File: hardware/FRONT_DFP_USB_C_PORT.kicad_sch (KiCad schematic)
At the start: 26 parts, among them J5 USB4200-03-A (VIRT FLAG MOUNT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, Q18 PMOS, Q19 PMOS, Q20 PMOS, Q21 PMOS

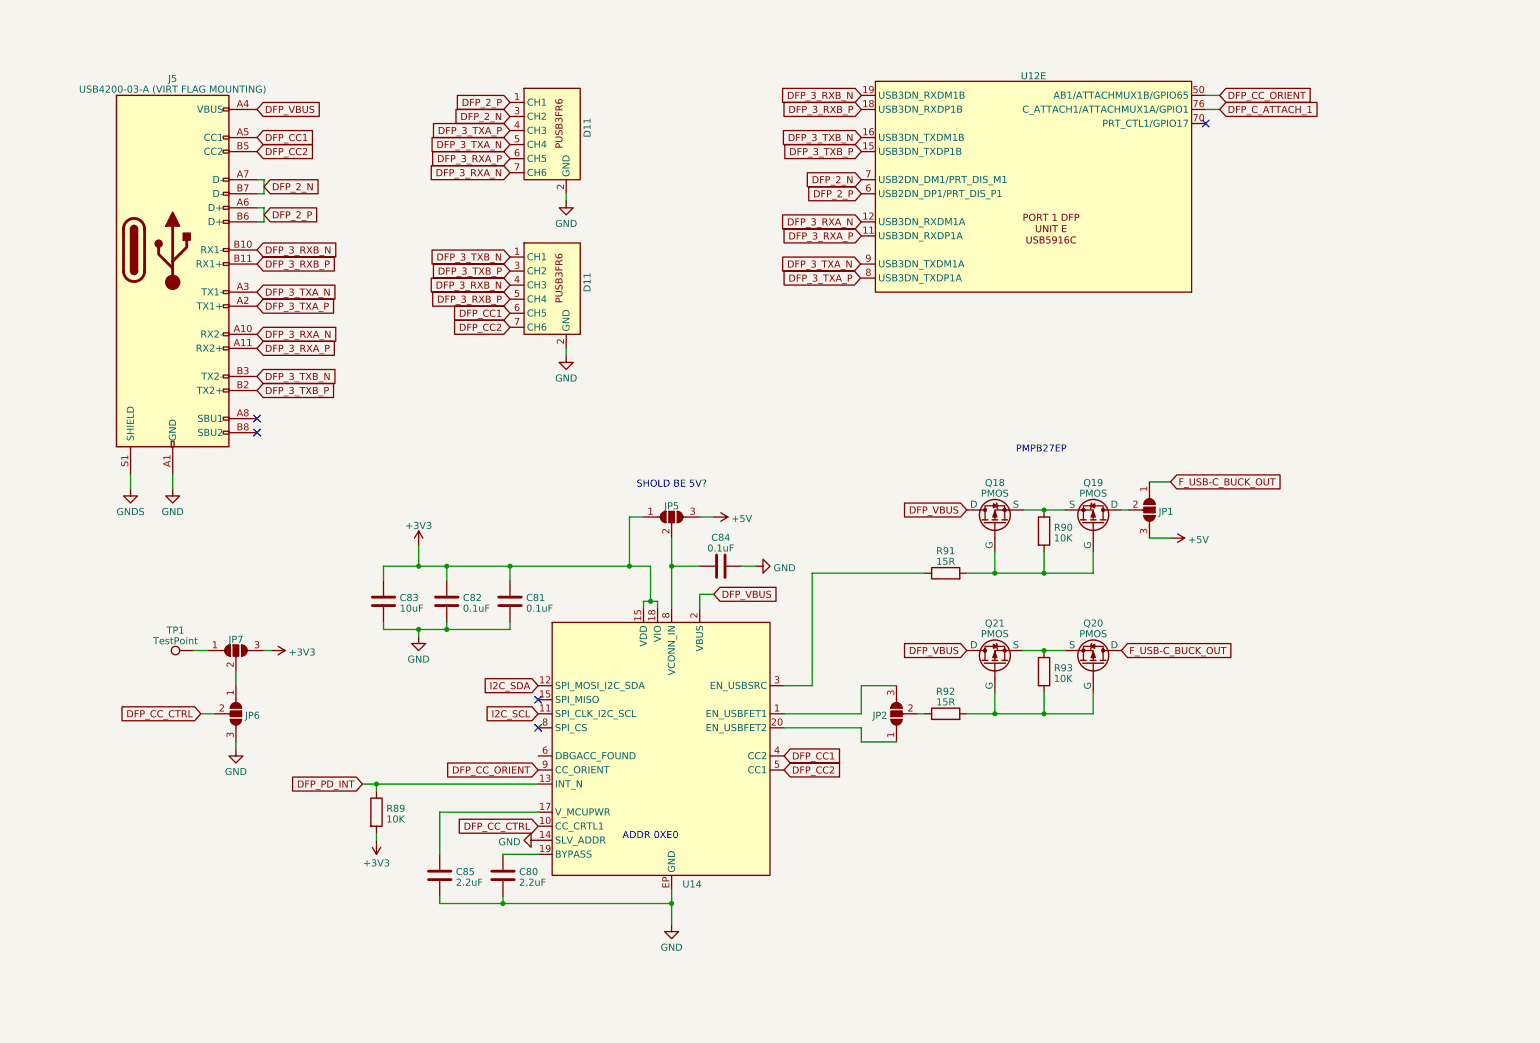
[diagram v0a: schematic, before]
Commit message: working on hardware
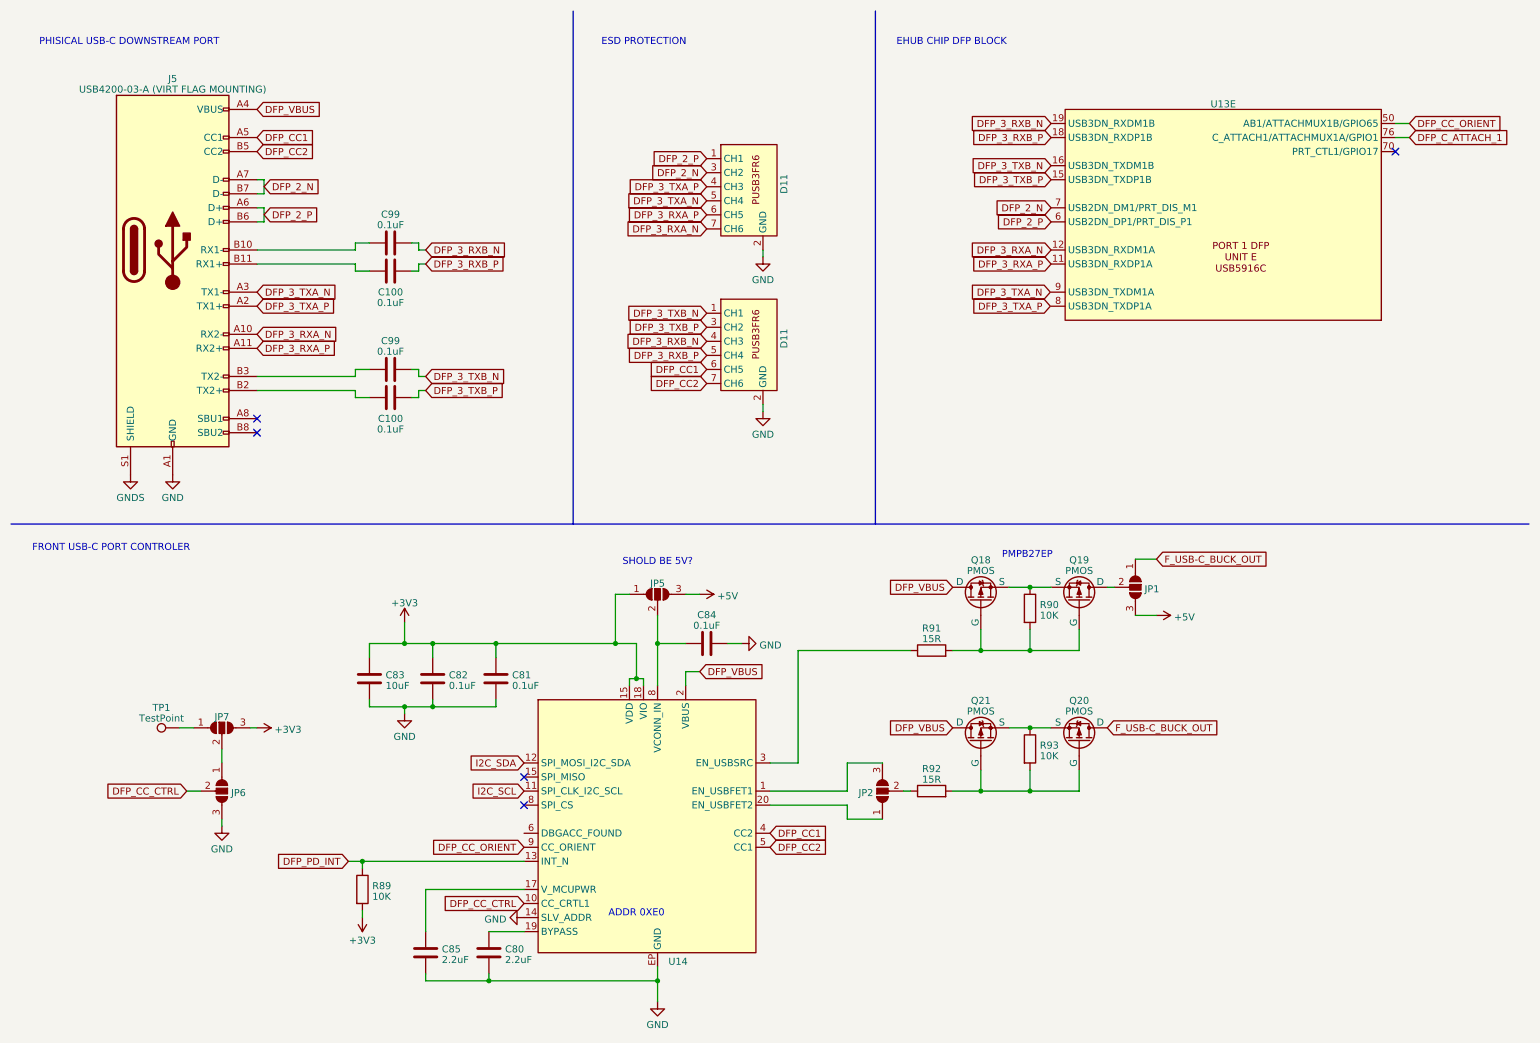
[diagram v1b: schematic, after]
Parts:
- added C100 (x2), C99 (x2): 0.1uF, Capacitor_SMD:C_0603_1608Metric, symbol Device:C
- C80, C81, C82, C83, C84, C85: footprint (none) -> Capacitor_SMD:C_0603_1608Metric
- JP1, JP2, JP5, JP6, JP7: footprint (none) -> Jumper:SolderJumper-3_P1.3mm_Open_RoundedPad1.0x1.5mm_NumberLabels
- Q18, Q19, Q20, Q21: footprint (none) -> CARTHING:TRANS_PMPB11EN_115
- TP1: footprint (none) -> TestPoint:TestPoint_Pad_D1.5mm
- renumbered U12 to U13
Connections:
- net DFP_3_RXB_N: now also C99.2; no longer J5.B10 (RX1-)
- net DFP_3_RXB_P: now also C100.1; no longer J5.B11 (RX1+)
- net DFP_3_TXB_N: now also C99.2; no longer J5.B3 (TX2-)
- net DFP_3_TXB_P: now also C100.1; no longer J5.B2 (TX2+)
- new net: C100.2, J5.B11 (RX1+)
- new net: C99.1, J5.B10 (RX1-)
- new net: C100.2, J5.B2 (TX2+)
- new net: C99.1, J5.B3 (TX2-)
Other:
- note added: "EHUB CHIP DFP BLOCK"
- note added: "ESD PROTECTION"
- note added: "FRONT USB-C PORT CONTROLER"
- note added: "PHISICAL USB-C DOWNSTREAM PORT"
- moved on the sheet: C80, C81, C82, C83, C84, C85, D11, JP1, JP2, JP5, JP6, JP7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

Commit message: working assighning footprints still
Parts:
- R89, R90, R91, R92, R93: footprint (none) -> Resistor_SMD:R_0603_1608Metric
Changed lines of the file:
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@@
       (effects (font (size 1.27 1.27)) (justify left))
     )
-    (property "Footprint" "" (at 193.802 144.78 90)
+    (property "Footprint" "Resistor_SMD:R_0603_1608Metric" (at 193.802 144.78 90)
       (effects (font (size 1.27 1.27)) hide)
     )
@@
       (effects (font (size 1.27 1.27)))
     )
-    (property "Footprint" "" (at 177.8 128.778 90)
+    (property "Footprint" "Resistor_SMD:R_0603_1608Metric" (at 177.8 128.778 90)
       (effects (font (size 1.27 1.27)) hide)
     )
@@
       (effects (font (size 1.27 1.27)) (justify left))
     )
-    (property "Footprint" "" (at 73.152 170.18 90)
+    (property "Footprint" "Resistor_SMD:R_0603_1608Metric" (at 73.152 170.18 90)
       (effects (font (size 1.27 1.27)) hide)
     )
@@
       (effects (font (size 1.27 1.27)))
     )
-    (property "Footprint" "" (at 177.8 154.178 90)
+    (property "Footprint" "Resistor_SMD:R_0603_1608Metric" (at 177.8 154.178 90)
       (effects (font (size 1.27 1.27)) hide)
     )
@@
       (effects (font (size 1.27 1.27)) (justify left))
     )
-    (property "Footprint" "" (at 193.802 119.38 90)
-      (effects (font (size 1.27 1.27)) hide)
-    )
+    (property "Footprint" "Resistor_SMD:R_0603_1608Metric" (at 193.802 119.38 90)
+      (effects (font (size 1.27 1.27)) hide)
+    )

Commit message: FINALY starting the pcb
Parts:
- D11: footprint (none) -> CARTHING:PUSB3AB6Z_NEX
- J5: footprint (none) -> CARTHING:USB4200-03-A_REVA
- U13: footprint (none) -> CARTHING:VQFN100_KD_MCH
- U14: footprint (none) -> CARTHING:PTN5100BSMP
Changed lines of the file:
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@@
       (effects (font (size 1.27 1.27)))
     )
-    (property "Footprint" "" (at 44.45 54.61 0)
+    (property "Footprint" "CARTHING:USB4200-03-A_REVA" (at 44.45 54.61 0)
       (effects (font (size 1.27 1.27)) hide)
     )
@@
       (effects (font (size 1.27 1.27)))
     )
-    (property "Footprint" "" (at 138.43 25.4 0)
+    (property "Footprint" "CARTHING:PUSB3AB6Z_NEX" (at 138.43 25.4 0)
       (effects (font (size 1.27 1.27)) hide)
     )
@@
       (effects (font (size 1.27 1.27)))
     )
-    (property "Footprint" "" (at 241.3 87.63 0)
+    (property "Footprint" "CARTHING:VQFN100_KD_MCH" (at 241.3 87.63 0)
       (effects (font (size 1.27 1.27)) hide)
     )
@@
       (effects (font (size 1.27 1.27)))
     )
-    (property "Footprint" "" (at 138.43 53.34 0)
+    (property "Footprint" "CARTHING:PUSB3AB6Z_NEX" (at 138.43 53.34 0)
       (effects (font (size 1.27 1.27)) hide)
     )
@@
       (effects (font (size 1.27 1.27)))
     )
-    (property "Footprint" "" (at 102.87 127 0)
-      (effects (font (size 1.27 1.27)) hide)
-    )
+    (property "Footprint" "CARTHING:PTN5100BSMP" (at 102.87 127 0)
+      (effects (font (size 1.27 1.27)) hide)
+    )
